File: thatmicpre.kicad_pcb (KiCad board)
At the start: 2 copper layers, 38.5 x 24 mm, 12 parts, among them J1 Conn_01x07_Female, U1 THAT1512

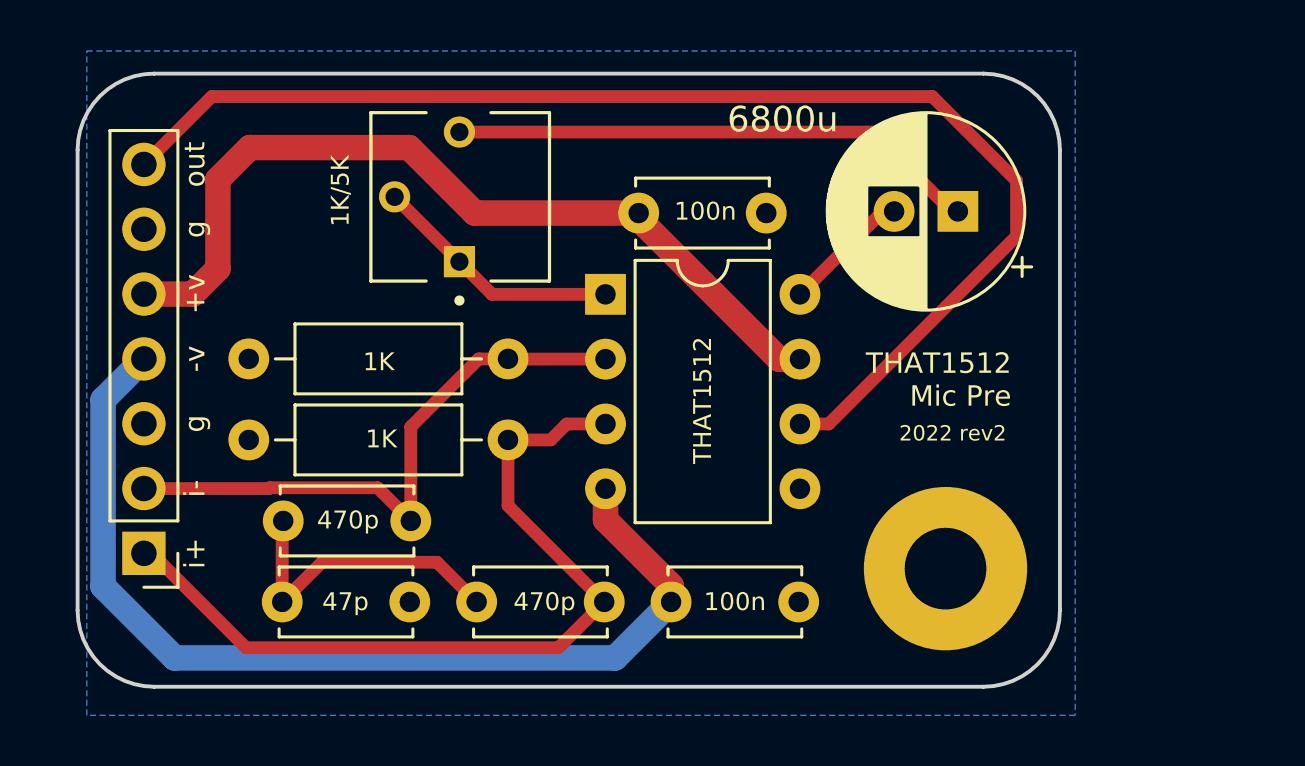
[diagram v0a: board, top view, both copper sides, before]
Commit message: change C6 footprint
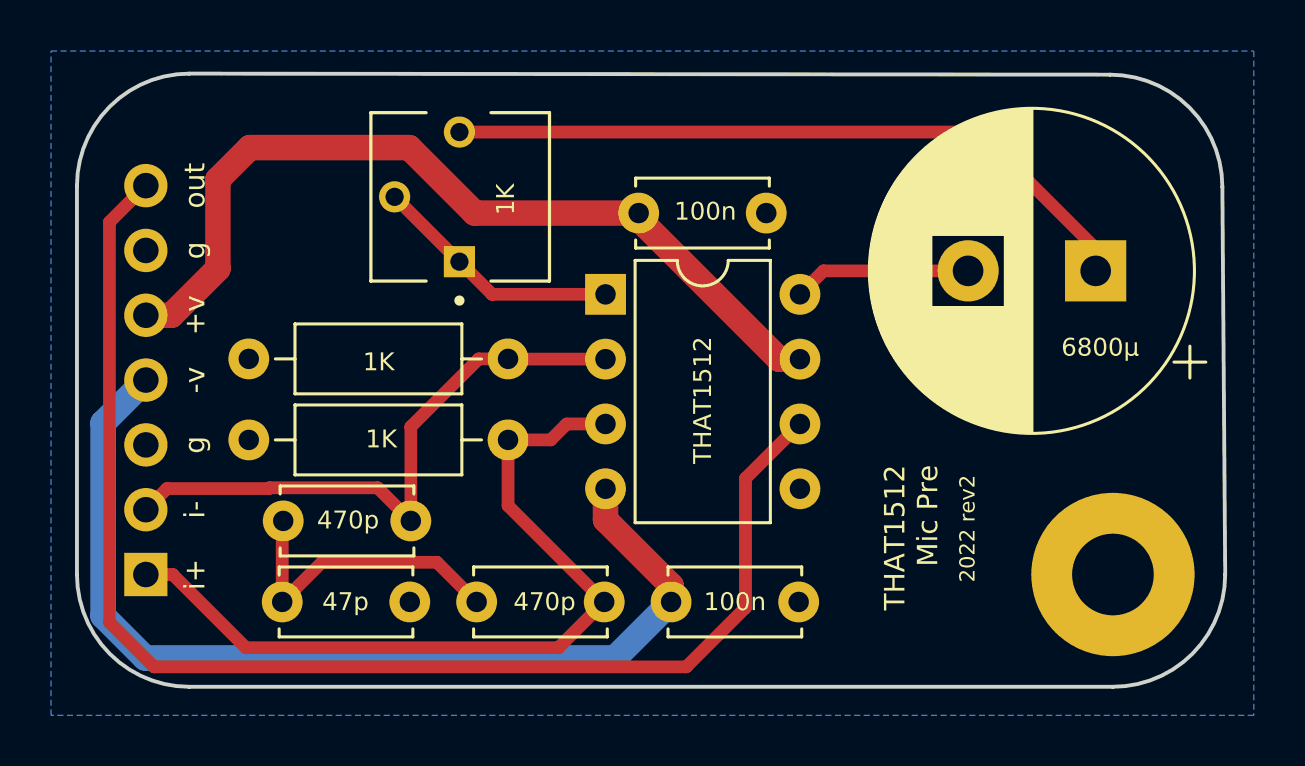
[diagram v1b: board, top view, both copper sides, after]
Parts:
- C6: value 6800u -> 6800μ; footprint Capacitor_THT:CP_Radial_D7.5mm_P2.50mm -> Capacitor_THT:CP_Radial_D12.5mm_P5.00mm
- RV1: value 1K/5K -> 1K
- moved H4 6.56 mm to (125.0, 72.4)
- moved C6 5.88 mm to (124.3, 60.5)
- moved J1 0.83 mm to (87.1, 72.4)
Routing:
- net Net-(RV1-Pad3): track 20.8 -> 27.7 mm
- net Out: track 50.4 -> 52.4 mm
- net Net-(U1-Pad8): track 5.04 -> 6.97 mm
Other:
- board size 38.5 x 24 mm -> 45 x 24 mm
